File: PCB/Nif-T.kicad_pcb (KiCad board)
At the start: 2 copper layers, 100 x 100 mm, 0 parts

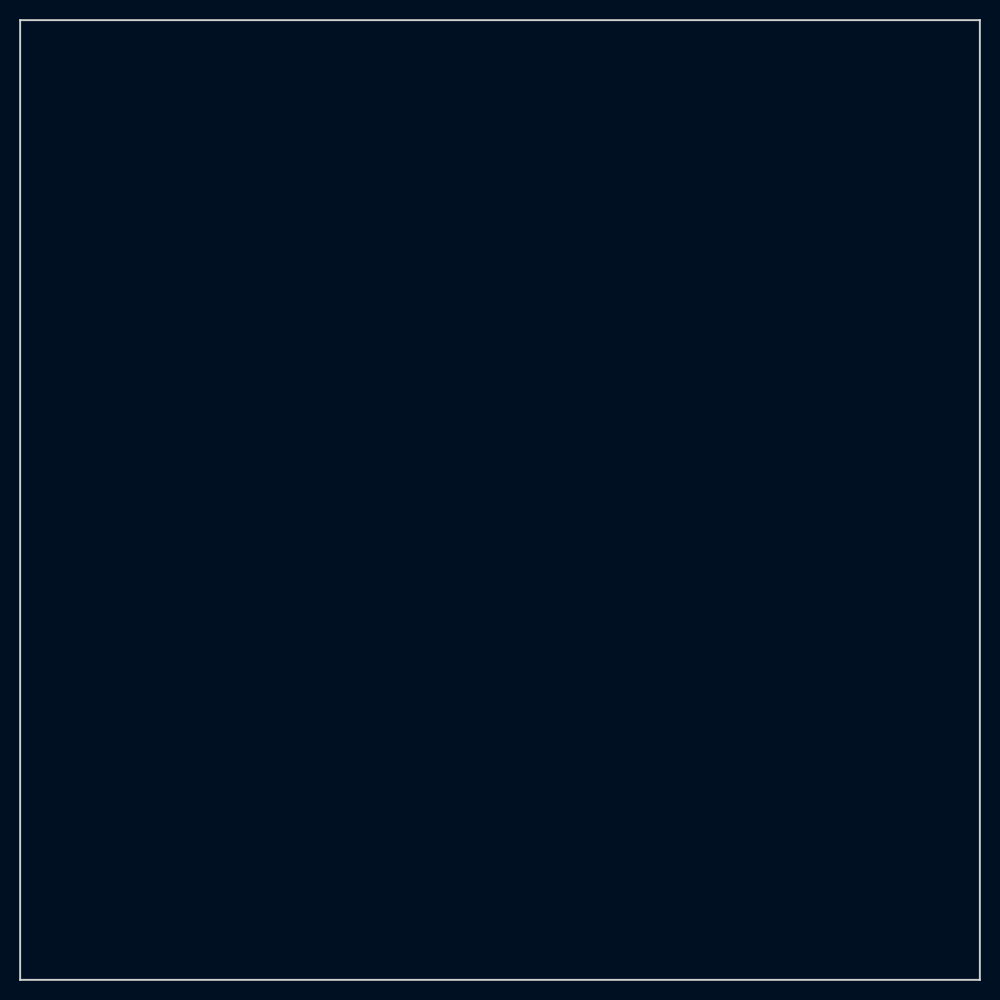
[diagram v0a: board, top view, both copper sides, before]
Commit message: PCB Reconfigured and Rerouted
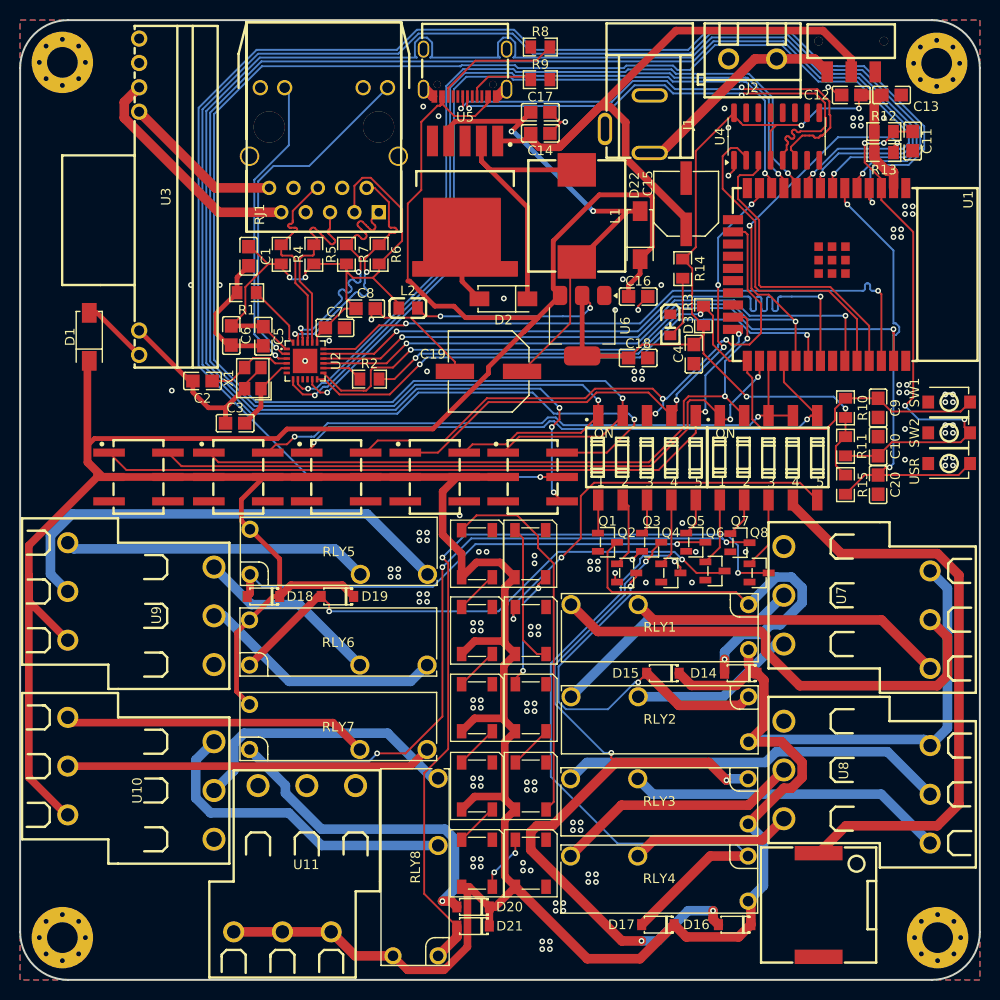
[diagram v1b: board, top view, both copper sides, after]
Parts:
- added BUZZER1: FST-1230, imported_components:BUZ-SMD_L12.0-W12.0_FUET-1230, F.Cu at (233.2, 142.2)
- added C1: 0.22uF, imported_components:C0805, F.Cu at (173.8, 74.6)
- added C10: 0.1uF, imported_components:C0805, F.Cu at (239.4, 94.4)
- added C11: 1uF, imported_components:C0805, F.Cu at (243.0, 62.6)
- added C12: 10uF, imported_components:C0805, F.Cu at (236.6, 57.8)
- added C13: 0.1uF, imported_components:C0805, F.Cu at (240.8, 57.8)
- added C14: 10uF, imported_components:C0805, F.Cu at (204.2, 61.8)
- added C15: RVT1H470M0607, imported_components:CAP-SMD_BD6.3-L6.6-W6.6-LS7.6-FD, F.Cu at (219.4, 69.1)
- added C16: 10uF, imported_components:C0805, F.Cu at (214.4, 78.8)
- added C17: 10uF, imported_components:C0805, F.Cu at (204.2, 59.6)
- added C18: 10uF, imported_components:C0805, F.Cu at (214.4, 85.2)
- added C19: RVT1E331M0810, imported_components:CAP-SMD_BD8.0-L8.3-W8.3-LS9.3-FD-1, F.Cu at (198.8, 86.6)
- added C2: 0.22uF, imported_components:C0805, F.Cu at (169.0, 87.6)
- added C20: 0.1uF, imported_components:C0805, F.Cu at (239.4, 98.4)
- added C3: 0.22uF, imported_components:C0805, F.Cu at (172.4, 92.0)
- added C4: 0.1uF, imported_components:C0805, F.Cu at (220.2, 84.8)
- added C5: 0.1uF, imported_components:C0805, F.Cu at (175.3, 82.9)
- added C6: 1uF, imported_components:C0805, F.Cu at (172.0, 82.9)
- added C7: 0.1uF, imported_components:C0805, F.Cu at (182.8, 82.1)
- added C8: 1uF, imported_components:C0805, F.Cu at (186.0, 80.1)
- added C9: 0.1uF, imported_components:C0805, F.Cu at (239.4, 90.4)
- added D1: SS54_C22452, imported_components:SMA_L4.4-W2.8-LS5.4-R-RD, F.Cu at (157.2, 83.0)
- added D10: SK6812, LED_SMD:LED_SK6812_PLCC4_5.0x5.0mm_P3.2mm, F.Cu at (197.6, 121.7)
- added D11: SK6812, LED_SMD:LED_SK6812_PLCC4_5.0x5.0mm_P3.2mm, F.Cu at (197.6, 129.8)
- added D12: SK6812, LED_SMD:LED_SK6812_PLCC4_5.0x5.0mm_P3.2mm, F.Cu at (197.6, 137.8)
- added D13: SK6812, LED_SMD:LED_SK6812_PLCC4_5.0x5.0mm_P3.2mm, F.Cu at (203.2, 137.8)
- added D14: 1N4148W-E3-08, new_imported_components:SOD-123_L2.8-W1.8-LS3.7-RD, F.Cu at (225.1, 118.0)
- added D15: 1N4148W-E3-08, new_imported_components:SOD-123_L2.8-W1.8-LS3.7-RD, F.Cu at (217.0, 118.0)
- added D16: 1N4148W-E3-08, new_imported_components:SOD-123_L2.8-W1.8-LS3.7-RD, F.Cu at (224.4, 144.2)
- added D17: 1N4148W-E3-08, new_imported_components:SOD-123_L2.8-W1.8-LS3.7-RD, F.Cu at (216.4, 144.2)
- added D18: 1N4148W-E3-08, new_imported_components:SOD-123_L2.8-W1.8-LS3.7-RD, F.Cu at (175.3, 110.0)
- added D19: 1N4148W-E3-08, new_imported_components:SOD-123_L2.8-W1.8-LS3.7-RD, F.Cu at (183.1, 110.0)
- added D2: SS54_C22452, imported_components:SMA_L4.4-W2.8-LS5.4-R-RD, F.Cu at (200.4, 79.0)
- added D20: 1N4148W-E3-08, new_imported_components:SOD-123_L2.8-W1.8-LS3.7-RD, F.Cu at (197.2, 142.4)
- added D21: 1N4148W-E3-08, new_imported_components:SOD-123_L2.8-W1.8-LS3.7-RD, F.Cu at (197.2, 144.4)
- added D22: SS54_C22452, imported_components:SMA_L4.4-W2.8-LS5.4-R-RD, F.Cu at (214.6, 72.4)
- added D3: LED, imported_components:LED0805-RD, F.Cu at (217.8, 81.8)
- added D4: SK6812, LED_SMD:LED_SK6812_PLCC4_5.0x5.0mm_P3.2mm, F.Cu at (203.2, 113.6)
- added D5: SK6812, LED_SMD:LED_SK6812_PLCC4_5.0x5.0mm_P3.2mm, F.Cu at (203.2, 105.6)
- added D6: SK6812, LED_SMD:LED_SK6812_PLCC4_5.0x5.0mm_P3.2mm, F.Cu at (203.2, 121.7)
- added D7: SK6812, LED_SMD:LED_SK6812_PLCC4_5.0x5.0mm_P3.2mm, F.Cu at (203.2, 129.8)
- added D8: SK6812, LED_SMD:LED_SK6812_PLCC4_5.0x5.0mm_P3.2mm, F.Cu at (197.6, 105.6)
- added D9: SK6812, LED_SMD:LED_SK6812_PLCC4_5.0x5.0mm_P3.2mm, F.Cu at (197.6, 113.6)
- added H1: MountingHole, MountingHole:MountingHole_3.2mm_M3_Pad_Via, F.Cu at (154.4, 54.4)
- added H2: MountingHole, MountingHole:MountingHole_3.2mm_M3_Pad_Via, F.Cu at (245.5, 54.5)
- added H3: MountingHole, MountingHole:MountingHole_3.2mm_M3_Pad_Via, F.Cu at (154.4, 145.6)
- added H4: MountingHole, MountingHole:MountingHole_3.2mm_M3_Pad_Via, F.Cu at (245.6, 145.6)
- added J1: Barrel_Jack, imported_components:DC-IN-TH_DC-005-A200, F.Cu at (213.3, 60.8)
- added J2: Conn_01x02, imported_components:CONN-TH_P5.00_KF301-5.0-2P, F.Cu at (226.3, 54.0)
- added J3: Conn_02x03_Odd_Even, imported_components:HDR-SMD_6P-P2.54-V, F.Cu at (162.2, 99.0)
- added J4: Conn_02x03_Odd_Even, imported_components:HDR-SMD_6P-P2.54-V, F.Cu at (172.6, 99.0)
- added J5: Conn_02x03_Odd_Even, imported_components:HDR-SMD_6P-P2.54-V, F.Cu at (182.8, 99.0)
- added J6: Conn_02x03_Odd_Even, imported_components:HDR-SMD_6P-P2.54-V, F.Cu at (193.1, 99.0)
- added J7: Conn_02x03_Odd_Even, imported_components:HDR-SMD_6P-P2.54-V, F.Cu at (203.3, 99.0)
- added L1: CYA1040-33UH, imported_components:IND-SMD_L11.6-W10.1, F.Cu at (208.0, 70.4)
- added L2: BLM21PG221SN1D, new_imported_components:L0805, F.Cu at (190.4, 80.0)
- added P1: USB_C_Plug, imported_components:USB-C_SMD-TYPE-C-31-M-12, F.Cu at (196.4, 55.5)
- added Q1: S8050, new_imported_components:SOT-23-3_L2.9-W1.3-P1.90-LS2.4-BR, F.Cu at (211.2, 104.4)
- added Q2: S8050, new_imported_components:SOT-23-3_L2.9-W1.3-P1.90-LS2.4-BR, F.Cu at (213.2, 107.6)
- added Q3: S8050, new_imported_components:SOT-23-3_L2.9-W1.3-P1.90-LS2.4-BR, F.Cu at (215.8, 104.4)
- added Q4: S8050, new_imported_components:SOT-23-3_L2.9-W1.3-P1.90-LS2.4-BR, F.Cu at (217.8, 107.6)
- added Q5: S8050, new_imported_components:SOT-23-3_L2.9-W1.3-P1.90-LS2.4-BR, F.Cu at (220.4, 104.4)
- added Q6: S8050, new_imported_components:SOT-23-3_L2.9-W1.3-P1.90-LS2.4-BR, F.Cu at (222.4, 107.4)
- added Q7: S8050, new_imported_components:SOT-23-3_L2.9-W1.3-P1.90-LS2.4-BR, F.Cu at (225.0, 104.5)
- added Q8: S8050, new_imported_components:SOT-23-3_L2.9-W1.3-P1.90-LS2.4-BR, F.Cu at (227.0, 107.6)
- added R1: 12.1k, imported_components:R0805, F.Cu at (173.6, 78.4)
- added R10: 10k, imported_components:R0805, F.Cu at (236.0, 90.4)
- added R11: 10k, imported_components:R0805, F.Cu at (236.0, 94.4)
- added R12: 10k, imported_components:R0805, F.Cu at (240.0, 61.6)
- added R13: 10k, imported_components:R0805, F.Cu at (240.0, 63.8)
- added R14: 200, imported_components:R0805, F.Cu at (219.0, 75.9)
- added R15: 10k, imported_components:R0805, F.Cu at (236.0, 98.4)
- added R2: 22, imported_components:R0805, F.Cu at (186.4, 87.4)
- added R3: 10k, imported_components:R0805, F.Cu at (221.2, 80.8)
- added R4: 49.9, imported_components:R0805, F.Cu at (177.2, 74.4)
- added R5: 49.9, imported_components:R0805, F.Cu at (180.6, 74.4)
- added R6: 49.9, imported_components:R0805, F.Cu at (187.4, 74.4)
- added R7: 49.9, imported_components:R0805, F.Cu at (184.0, 74.4)
- added R8: 5.1k, imported_components:R0805, F.Cu at (204.2, 52.8)
- added R9: 5.1k, imported_components:R0805, F.Cu at (204.2, 56.2)
- added RJ1: HY931147C, new_imported_components:RJ45-TH_HY931147C, F.Cu at (181.7, 63.5)
- added RLY1: G5NB-1A-E-DC5V, new_imported_components:RELAY-TH_G5NB-1A-E-DCXX, F.Cu at (216.7, 113.2)
- added RLY2: G5NB-1A-E-DC5V, new_imported_components:RELAY-TH_G5NB-1A-E-DCXX, F.Cu at (216.7, 122.8)
- added RLY3: G5NB-1A-E-DC5V, new_imported_components:RELAY-TH_G5NB-1A-E-DCXX, F.Cu at (216.6, 131.4)
- added RLY4: G5NB-1A-E-DC5V, new_imported_components:RELAY-TH_G5NB-1A-E-DCXX, F.Cu at (216.6, 139.4)
- added RLY5: G5NB-1A-E-DC5V, new_imported_components:RELAY-TH_G5NB-1A-E-DCXX, F.Cu at (183.2, 105.4)
- added RLY6: G5NB-1A-E-DC5V, new_imported_components:RELAY-TH_G5NB-1A-E-DCXX, F.Cu at (183.2, 114.8)
- added RLY7: G5NB-1A-E-DC5V, new_imported_components:RELAY-TH_G5NB-1A-E-DCXX, F.Cu at (183.2, 123.7)
- added RLY8: G5NB-1A-E-DC5V, new_imported_components:RELAY-TH_G5NB-1A-E-DCXX, F.Cu at (191.2, 138.2)
- added SW1: SW_Push, imported_components:SW-SMD_L3.9-W3.0-P4.45, F.Cu at (246.8, 89.8)
- added SW2: SW_Push, imported_components:SW-SMD_L3.9-W3.0-P4.45, F.Cu at (246.8, 93.0)
- added SW3: SW_Push, imported_components:SW-SMD_L3.9-W3.0-P4.45, F.Cu at (246.8, 96.2)
- added SW4: SW_SPDT, imported_components:SW-SMD_MST-12D18G4-SPDT-SLIDE-SWITCH, F.Cu at (236.6, 55.4)
- added SW5: DSIC-05-LS-GER, new_imported_components:SW-SMD_DSIC-05-LS-GER, F.Cu at (228.0, 95.6)
- added SW6: DSIC-05-LS-GER, new_imported_components:SW-SMD_DSIC-05-LS-GER, F.Cu at (215.3, 95.6)
- added U1: ESP32-WROOM-32E(4MB), new_imported_components:WIFI-SMD_ESP32-WROOM-32E, F.Cu at (233.3, 76.5)
- added U10: DB128B-5.08-3P-BK-S, new_imported_components:CONN-TH_DB128B-5.08-3P-XX-S, F.Cu at (162.6, 129.0)
- added U11: DB128B-5.08-3P-BK-S, new_imported_components:CONN-TH_DB128B-5.08-3P-XX-S, F.Cu at (178.6, 137.4)
- added U2: LAN8720A-CP-TR, new_imported_components:QFN-24_L4.0-W4.0-P0.50-BL-EP2.6, F.Cu at (179.7, 85.5)
- added U3: DP1435-5V, new_imported_components:PWRM-TH_DP1435-XX, F.Cu at (162.4, 68.4)
- added U4: CH340C, Package_SO:SOIC-16_3.9x9.9mm_P1.27mm, F.Cu at (228.8, 62.1)
- added U5: LM2596SX-5.0/NOPB, imported_components:TO-263-5_L10.2-W8.9-P1.70-TL, F.Cu at (196.4, 67.6)
- added U6: AMS1117-3.3, Package_TO_SOT_SMD:SOT-223-3_TabPin2, F.Cu at (208.6, 81.8)
- added U7: DB128B-5.08-3P-BK-S, new_imported_components:CONN-TH_DB128B-5.08-3P-XX-S, F.Cu at (237.2, 111.2)
- added U8: DB128B-5.08-3P-BK-S, new_imported_components:CONN-TH_DB128B-5.08-3P-XX-S, F.Cu at (237.2, 129.4)
- added U9: DB128B-5.08-3P-BK-S, new_imported_components:CONN-TH_DB128B-5.08-3P-XX-S, F.Cu at (162.6, 110.8)
- added X1: X322525MOB4SI, new_imported_components:CRYSTAL-SMD_4P-L3.2-W2.5-BL, F.Cu at (174.2, 87.3)
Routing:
- net +5V: track 0.00 -> 529.0 mm
- net GPIO 33: track 0.00 -> 181.4 mm, vias 0 -> 2
- net GPIO 32: track 0.00 -> 181.1 mm, vias 0 -> 2
- net GPIO 37: track 0.00 -> 180.0 mm, vias 0 -> 2
- net GPIO 35: track 0.00 -> 179.7 mm, vias 0 -> 4
- net GPIO 36: track 0.00 -> 168.5 mm, vias 0 -> 2
- net +3.3V: track 0.00 -> 128.2 mm, vias 0 -> 6
- net Net-(D20-A): track 0.00 -> 106.0 mm, vias 0 -> 4
- net 8720RST: track 0.00 -> 89.9 mm, vias 0 -> 4
- net RXD0/MODE0: track 0.00 -> 86.6 mm, vias 0 -> 2
- net RXD1/MODE1: track 0.00 -> 86.6 mm, vias 0 -> 2
- net Net-(D16-A): track 0.00 -> 84.9 mm, vias 0 -> 5
- net Net-(D21-A): track 0.00 -> 83.4 mm, vias 0 -> 2
- net CRS_DV/MODE2: track 0.00 -> 83.1 mm, vias 0 -> 2
- net ETH_CLK: track 0.00 -> 78.8 mm, vias 0 -> 2
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- added copper zone on B.Cu, net GND
- added copper zone on F.Cu, net GND
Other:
- outline, holes or cut-outs redrawn
- board text added: "USR"
